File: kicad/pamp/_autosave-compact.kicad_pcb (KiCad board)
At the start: 2 copper layers, 88 x 100 mm, 71 parts, among them J1 input, J2 output, J3 power, Q1 BC560C, Q10 MJE340, Q11 2SC4793, Q12 Q_PNP_BCE, Q13 MJL3281, Q14 MJL1302, Q2 2SA1381F, Q3 2SA1381F, Q5 BC560C, Q6 BC546B, Q8 2SC3503F, Q9 2SA1381F

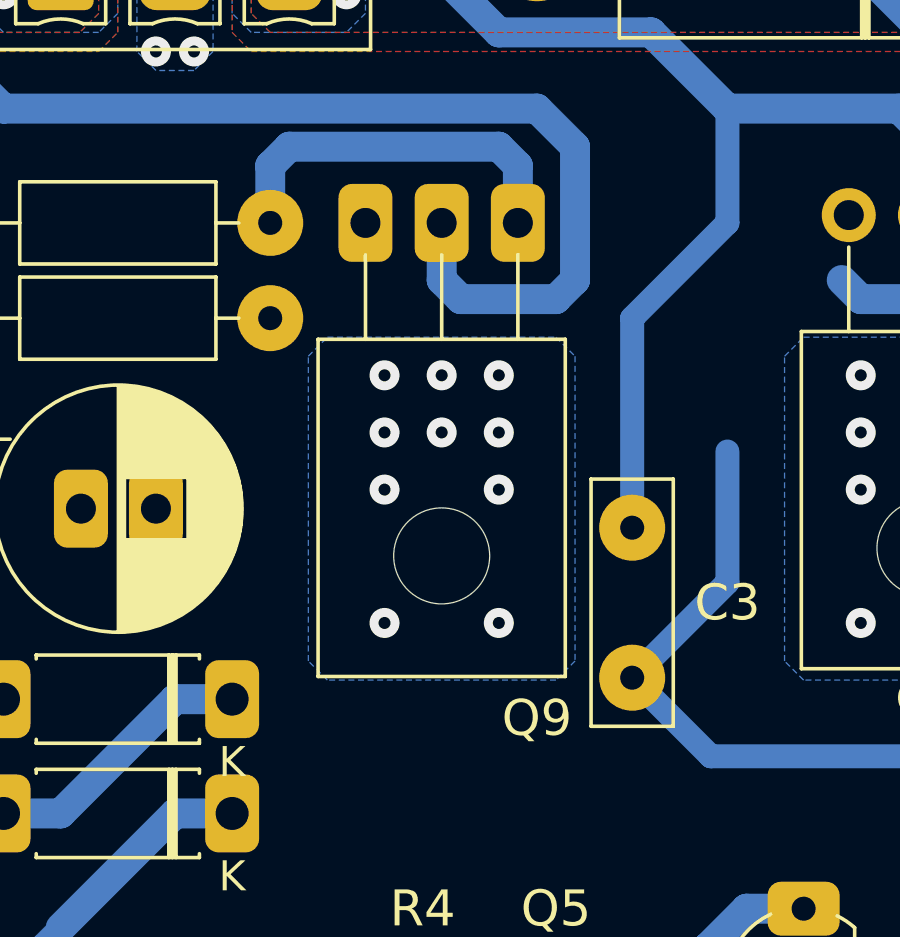
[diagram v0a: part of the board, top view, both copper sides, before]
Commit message: feat: project organization
Signed-off-by: Nenad Radulovic <nenad.b.radulovic@gmail.com>
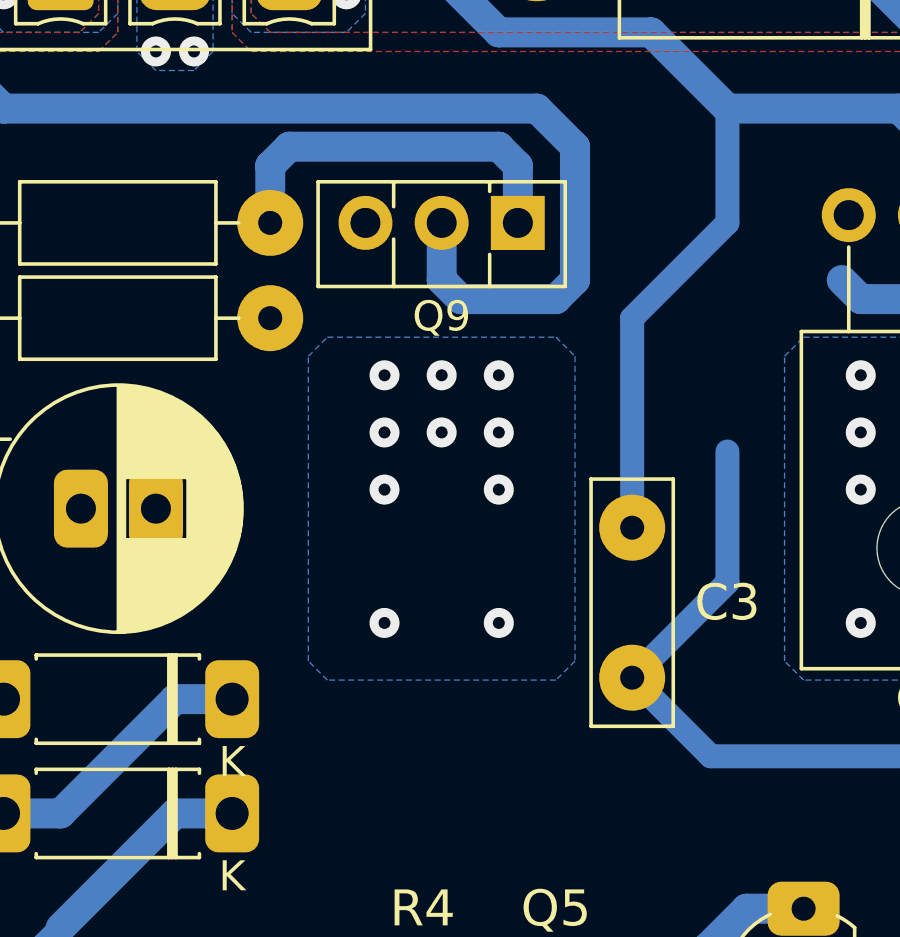
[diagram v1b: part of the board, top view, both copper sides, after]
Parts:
- Q9: footprint Package_TO_SOT_THT:TO-126-3_Horizontal_TabDown -> Package_TO_SOT_THT:TO-126-3_Vertical
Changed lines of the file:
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@@
-    )
-  )
-  (module Package_TO_SOT_THT:TO-126-3_Horizontal_TabDown (layer F.Cu)
-    (at 121.43 78.26 180)
-    (descr "TO-126-3, Horizontal, RM 2.54mm, see https://www.diodes.com/assets/Package-Files/TO126.pdf")
-    (tags "TO-126-3 Horizontal RM 2.54mm")
-    (fp_text reference Q9 (at -0.635 -16.51 180) (layer F.SilkS)
-      (effects (font (size 1.2 1.2) (thickness 0.15)))
-    )
-    (fp_text value 2SA1381F (at 2.54 1.9 180) (layer F.Fab)
-      (effects (font (size 1 1) (thickness 0.15)))
-    )
-    (fp_line (start 6.79 -15.25) (end -1.71 -15.25) (layer F.CrtYd) (width 0.05))
-    (fp_line (start 6.79 1.15) (end 6.79 -15.25) (layer F.CrtYd) (width 0.05))
-    (fp_line (start -1.71 1.15) (end 6.79 1.15) (layer F.CrtYd) (width 0.05))
-    (fp_line (start -1.71 -15.25) (end -1.71 1.15) (layer F.CrtYd) (width 0.05))
-    (fp_line (start 5.08 -3.88) (end 5.08 -1.066) (layer F.SilkS) (width 0.12))
-    (fp_line (start 2.54 -3.88) (end 2.54 -1.066) (layer F.SilkS) (width 0.12))
-    (fp_line (start 0 -3.88) (end 0 -1.05) (layer F.SilkS) (width 0.12))
-    (fp_line (start 6.66 -15.12) (end 6.66 -3.88) (layer F.SilkS) (width 0.12))
-    (fp_line (start -1.58 -15.12) (end -1.58 -3.88) (layer F.SilkS) (width 0.12))
-    (fp_line (start -1.58 -15.12) (end 6.66 -15.12) (layer F.SilkS) (width 0.12))
-    (fp_line (start -1.58 -3.88) (end 6.66 -3.88) (layer F.SilkS) (width 0.12))
-    (fp_line (start 5.08 -4) (end 5.08 0) (layer F.Fab) (width 0.1))
-    (fp_line (start 2.54 -4) (end 2.54 0) (layer F.Fab) (width 0.1))
-    (fp_line (start 0 -4) (end 0 0) (layer F.Fab) (width 0.1))
-    (fp_line (start 6.54 -4) (end -1.46 -4) (layer F.Fab) (width 0.1))
-    (fp_line (start 6.54 -15) (end 6.54 -4) (layer F.Fab) (width 0.1))
-    (fp_line (start -1.46 -15) (end 6.54 -15) (layer F.Fab) (width 0.1))
-    (fp_line (start -1.46 -4) (end -1.46 -15) (layer F.Fab) (width 0.1))
-    (fp_circle (center 2.54 -11.1) (end 4.14 -11.1) (layer F.Fab) (width 0.1))
-    (fp_text user %R (at 2.54 -16.12 180) (layer F.Fab)
-      (effects (font (size 1 1) (thickness 0.15)))
-    )
-    (pad "" np_thru_hole oval (at 2.54 -11.1 180) (size 3.2 3.2) (drill 3.2) (layers *.Cu *.Mask))
-    (pad 1 thru_hole roundrect (at 0 0 180) (size 1.8 2.6) (drill 1) (layers *.Cu *.Mask) (roundrect_rratio 0.25)
-      (net 19 "Net-(Q9-Pad1)"))
-    (pad 2 thru_hole roundrect (at 2.54 0 180) (size 1.8 2.6) (drill 1) (layers *.Cu *.Mask) (roundrect_rratio 0.25)
-      (net 12 "Net-(Q9-Pad2)"))
-    (pad 3 thru_hole roundrect (at 5.08 0 180) (size 1.8 2.6) (drill 1) (layers *.Cu *.Mask) (roundrect_rratio 0.25)
-      (net 36 "Net-(Q9-Pad3)"))
-    (model ${KISYS3DMOD}/Package_TO_SOT_THT.3dshapes/TO-126-3_Horizontal_TabDown.wrl
-      (at (xyz 0 0 0))
-      (scale (xyz 1 1 1))
-      (rotate (xyz 0 0 0))
     )
   )
@@
       (net 40 "Net-(C2-Pad2)"))
     (model ${KISYS3DMOD}/Capacitor_THT.3dshapes/CP_Radial_D8.0mm_P2.50mm.wrl
+      (at (xyz 0 0 0))
+      (scale (xyz 1 1 1))
+      (rotate (xyz 0 0 0))
+    )
+  )
+  (module Package_TO_SOT_THT:TO-126-3_Vertical (layer F.Cu)
+    (at 121.43 78.26 180)
+    (descr "TO-126-3, Vertical, RM 2.54mm, see https://www.diodes.com/assets/Package-Files/TO126.pdf")
+    (tags "TO-126-3 Vertical RM 2.54mm")
+    (fp_text reference Q9 (at 2.54 -3.12 180) (layer F.SilkS)
+      (effects (font (size 1 1) (thickness 0.15)))
+    )
+    (fp_text value 2SA1381F (at 2.54 2.5 180) (layer F.Fab)
+      (effects (font (size 1 1) (thickness 0.15)))
+    )
+    (fp_line (start -1.46 -2) (end -1.46 1.25) (layer F.Fab) (width 0.1))
+    (fp_line (start -1.46 1.25) (end 6.54 1.25) (layer F.Fab) (width 0.1))
+    (fp_line (start 6.54 1.25) (end 6.54 -2) (layer F.Fab) (width 0.1))
+    (fp_line (start 6.54 -2) (end -1.46 -2) (layer F.Fab) (width 0.1))
+    (fp_line (start 0.94 -2) (end 0.94 1.25) (layer F.Fab) (width 0.1))
+    (fp_line (start 4.14 -2) (end 4.14 1.25) (layer F.Fab) (width 0.1))
+    (fp_line (start -1.58 -2.12) (end 6.66 -2.12) (layer F.SilkS) (width 0.12))
+    (fp_line (start -1.58 1.37) (end 6.66 1.37) (layer F.SilkS) (width 0.12))
+    (fp_line (start -1.58 -2.12) (end -1.58 1.37) (layer F.SilkS) (width 0.12))
+    (fp_line (start 6.66 -2.12) (end 6.66 1.37) (layer F.SilkS) (width 0.12))
+    (fp_line (start 0.94 -2.12) (end 0.94 -1.05) (layer F.SilkS) (width 0.12))
+    (fp_line (start 0.94 1.05) (end 0.94 1.37) (layer F.SilkS) (width 0.12))
+    (fp_line (start 4.141 -2.12) (end 4.141 -0.54) (layer F.SilkS) (width 0.12))
+    (fp_line (start 4.141 0.54) (end 4.141 1.37) (layer F.SilkS) (width 0.12))
+    (fp_line (start -1.71 -2.25) (end -1.71 1.5) (layer F.CrtYd) (width 0.05))
+    (fp_line (start -1.71 1.5) (end 6.79 1.5) (layer F.CrtYd) (width 0.05))
+    (fp_line (start 6.79 1.5) (end 6.79 -2.25) (layer F.CrtYd) (width 0.05))
+    (fp_line (start 6.79 -2.25) (end -1.71 -2.25) (layer F.CrtYd) (width 0.05))
+    (fp_text user %R (at 2.54 -3.12 180) (layer F.Fab)
+      (effects (font (size 1 1) (thickness 0.15)))
+    )
+    (pad 1 thru_hole rect (at 0 0 180) (size 1.8 1.8) (drill 1) (layers *.Cu *.Mask)
+      (net 19 "Net-(Q9-Pad1)"))
+    (pad 2 thru_hole oval (at 2.54 0 180) (size 1.8 1.8) (drill 1) (layers *.Cu *.Mask)
+      (net 12 "Net-(Q9-Pad2)"))
+    (pad 3 thru_hole oval (at 5.08 0 180) (size 1.8 1.8) (drill 1) (layers *.Cu *.Mask)
+      (net 36 "Net-(Q9-Pad3)"))
+    (model ${KISYS3DMOD}/Package_TO_SOT_THT.3dshapes/TO-126-3_Vertical.wrl
       (at (xyz 0 0 0))
       (scale (xyz 1 1 1))
@@
   (segment (start 111.905 120.805) (end 110.635 119.535) (width 0.8) (layer B.Cu) (net 40))
   (segment (start 123.335 123.345) (end 122.065 122.075) (width 0.8) (layer B.Cu) (net 27))
-  (segment (start 110.945 123.035) (end 108.73 123.035) (width 0.8) (layer B.Cu) (net 27))
+  (segment (start 110.945 123.035) (end 108.73 123.035) (width 0.8) (layer B.Cu) (net 27) (status 20))
   (segment (start 123.335 126.52) (end 123.335 123.345) (width 0.8) (layer B.Cu) (net 27) (status 10))
   (segment (start 111.905 122.075) (end 110.945 123.035) (width 0.8) (layer B.Cu) (net 27))
